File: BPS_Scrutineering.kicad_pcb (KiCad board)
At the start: 2 copper layers, 77.5 x 64.8 mm, 26 parts, among them J1 Conn_01x01_Female, J10 Conn_01x01_Female, J11 Conn_01x01_Female, J12 Conn_01x01_Female, J13 Conn_01x01_Female, J14 Conn_01x01_Female, J2 Conn_01x01_Female, J3 Conn_01x01_Female, J4 Conn_01x01_Female, J5 Conn_01x01_Female, J6 Conn_01x01_Female, J7 Conn_01x01_Female, J8 Conn_01x01_Female, J9 Conn_01x01_Female, SW1 SW_DIP_x07, SW2 SW_DIP_x07

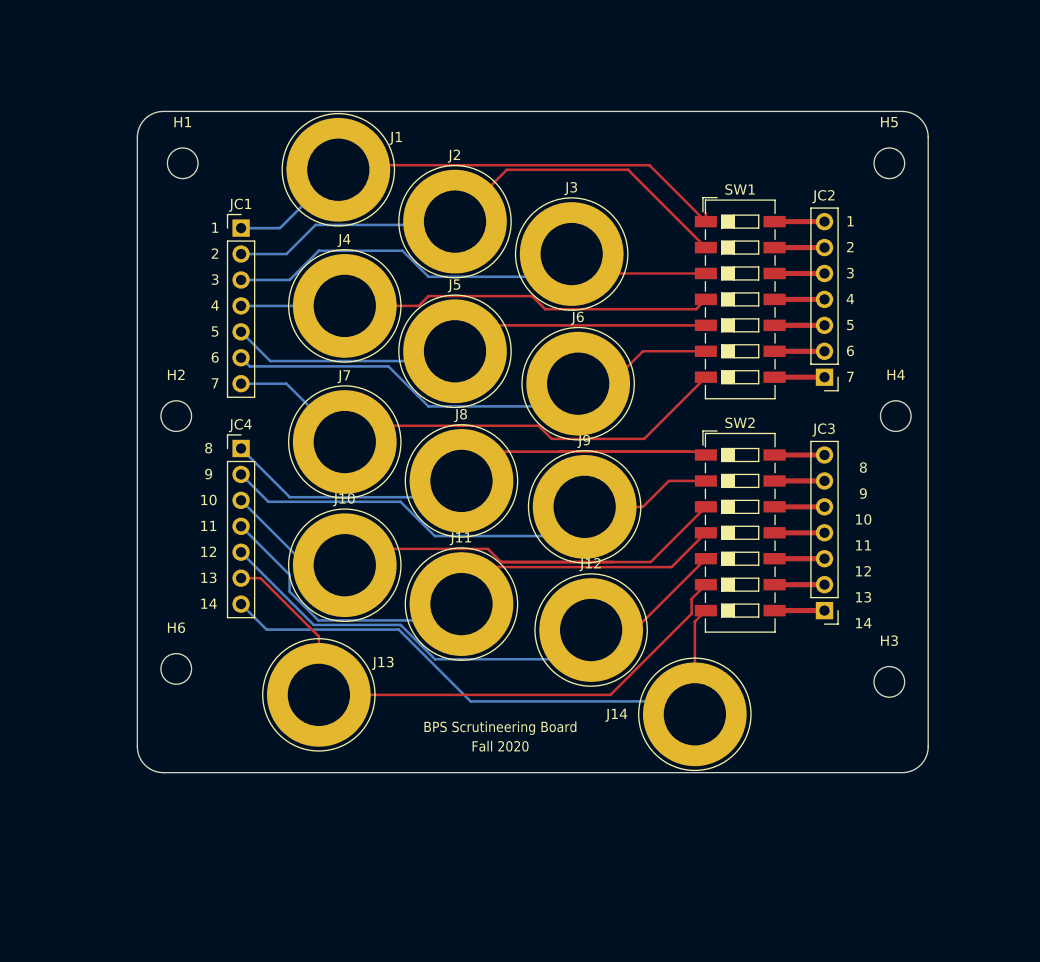
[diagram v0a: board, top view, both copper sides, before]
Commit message: Finished PCB
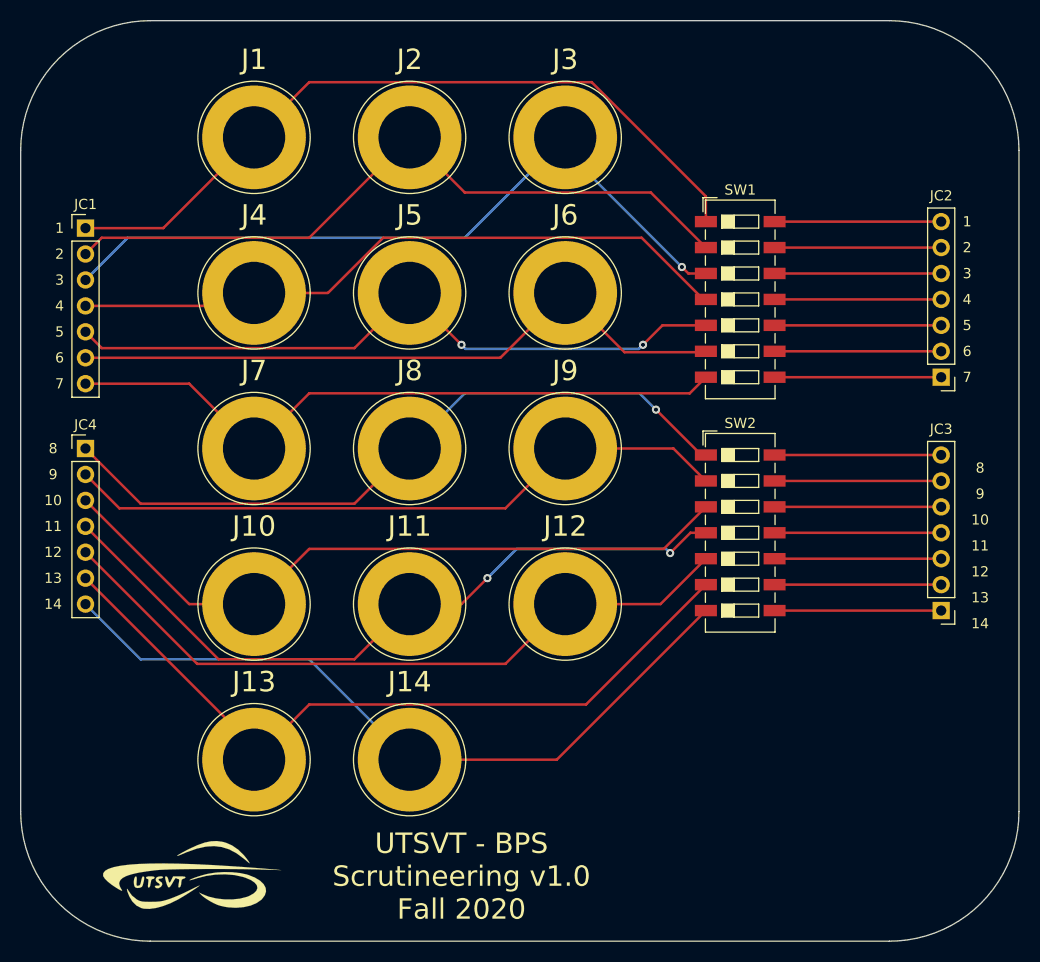
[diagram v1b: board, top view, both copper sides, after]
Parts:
- removed H1, H2, H3, H4, H5, H6: MountingHole, MountingHole:MountingHole_3mm
- added LOGO1: Logo_Placeholder, UTSVT_Special:UTSVT_Logo_Symbol, F.Cu at (85.1, 124.5)
- added LOGO2: Logo_Placeholder, UTSVT_Special:Hallock_Image, B.Cu at (139.7, 106.7)
- moved J14 28.3 mm to (106.7, 113.0)
- moved JC1 15.2 mm to (74.9, 61.0)
- moved JC4 15.2 mm to (74.9, 82.5)
- moved J3 11.4 mm to (121.9, 52.1)
- moved JC2 11.4 mm to (158.8, 75.6)
- moved JC3 11.4 mm to (158.8, 98.4)
- moved J10 9.67 mm to (91.4, 97.8)
- moved J2 9.38 mm to (106.7, 52.1)
- moved J13 8.98 mm to (91.4, 113.0)
- moved J4 8.98 mm to (91.4, 67.3)
- moved J6 8.98 mm to (121.9, 67.3)
- moved J7 8.91 mm to (91.4, 82.5)
- moved J1 8.84 mm to (91.4, 52.1)
- moved J5 7.24 mm to (106.7, 67.3)
- moved J9 6.02 mm to (121.9, 82.5)
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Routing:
- net Net-(J3-Pad1): track 49.5 -> 72.8 mm, vias 0 -> 1
- net Net-(J1-Pad1): track 51.2 -> 73.8 mm
- net Net-(J4-Pad1): track 46.9 -> 66.0 mm
- net Net-(J5-Pad1): track 48.2 -> 66.9 mm, vias 0 -> 2
- net Net-(J2-Pad1): track 52.1 -> 70.0 mm
- net Net-(J6-Pad1): track 49.7 -> 65.8 mm
- net Net-(J13-Pad1): track 60.3 -> 76.0 mm
- net Net-(J9-Pad1): track 50.3 -> 65.9 mm
- net Net-(J12-Pad1): track 54.0 -> 69.6 mm
- net Net-(J7-Pad1): track 51.6 -> 66.3 mm
- net Net-(J11-Pad1): track 59.1 -> 71.6 mm, vias 0 -> 2
- net Net-(J14-Pad1): track 61.1 -> 73.1 mm
- net Net-(JC3-Pad7): track 4.89 -> 16.3 mm
- net Net-(JC3-Pad6): track 4.89 -> 16.3 mm
- net Net-(JC3-Pad5): track 4.89 -> 16.3 mm
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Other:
- board size 77.5 x 64.8 mm -> 97.8 x 90.2 mm
- board text added: "UTSVT - BPS Scrutineering v1.0 Fall 2020"
- board text removed: "BPS Scrutineering Board"
- board text removed: "Fall 2020"
